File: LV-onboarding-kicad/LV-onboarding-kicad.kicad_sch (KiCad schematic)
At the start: 7 parts, among them J1 Current Transducer HASS 50 ..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, J2 AiM Sports Pressure Sensors X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, U1 NE555D, U2 ${SIM.PARAMS}, U3 ${SIM.PARAMS}

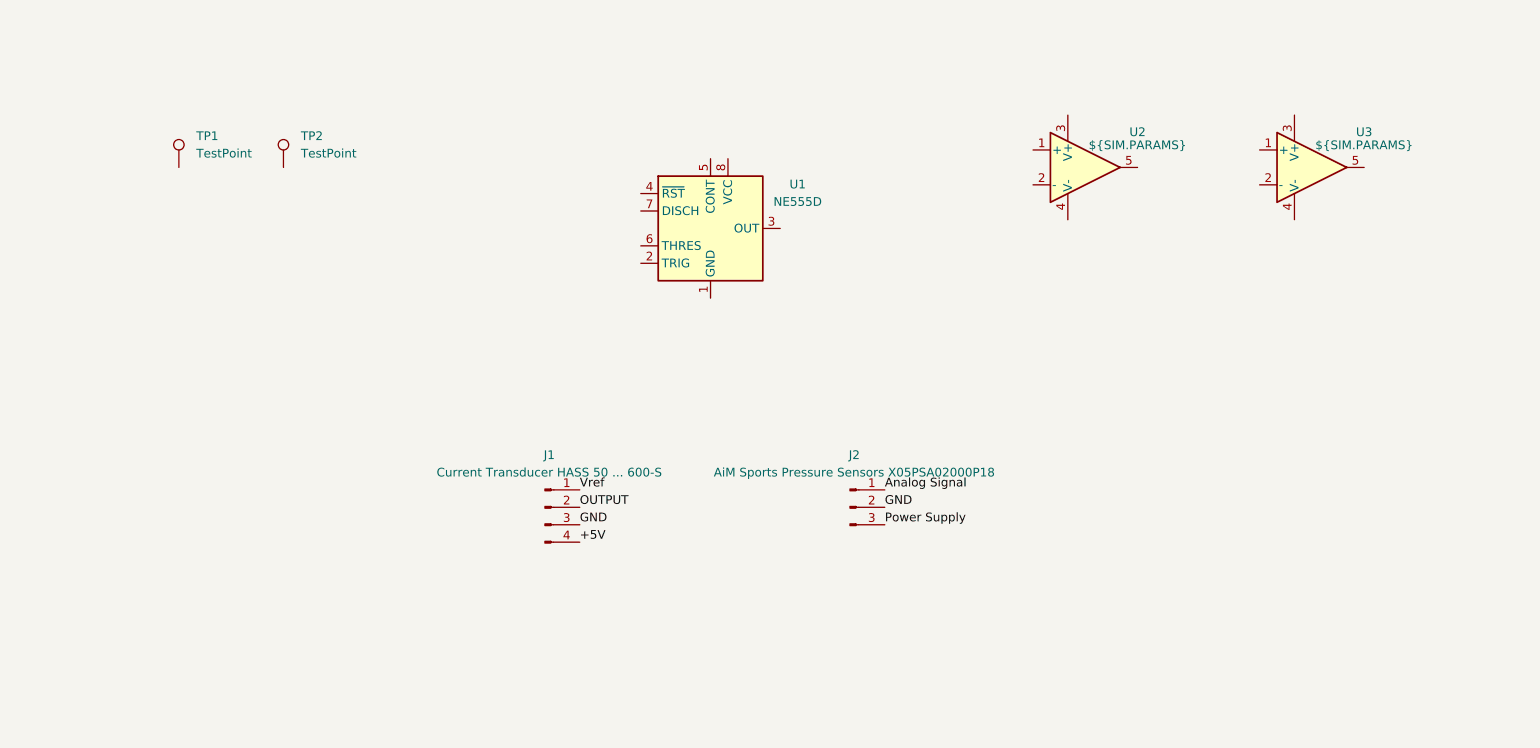
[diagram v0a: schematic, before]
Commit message: kicad
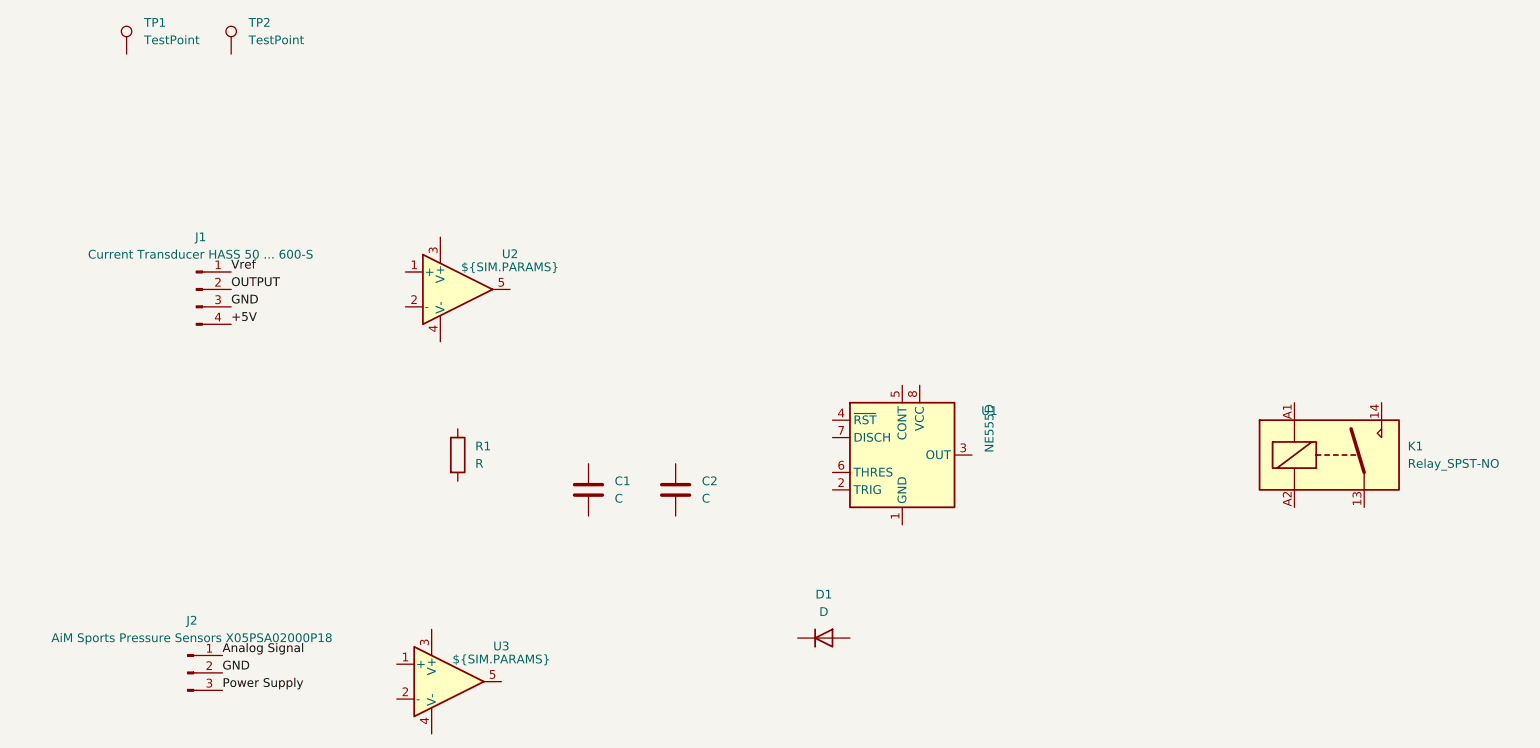
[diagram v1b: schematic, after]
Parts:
- added C1, C2: C, Package_SO:SOIC-8_3.9x4.9mm_P1.27mm, symbol Device:C
- added D1: D, symbol Device:D
- added K1: Relay_SPST-NO, Relay_THT:Relay_NCR_HHG1D-1, symbol Relay:Relay_SPST-NO
- added R1: R, Package_DIP:DIP-8_W7.62mm, symbol Device:R
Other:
- moved on the sheet: J1, J2, TP1, TP2, U1, U2, U3
